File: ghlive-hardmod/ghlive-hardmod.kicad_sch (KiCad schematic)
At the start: 8 parts, among them IC1 LDL212D33R, J1 Conn_01x02, U2 ESP32-S3-WROOM-1

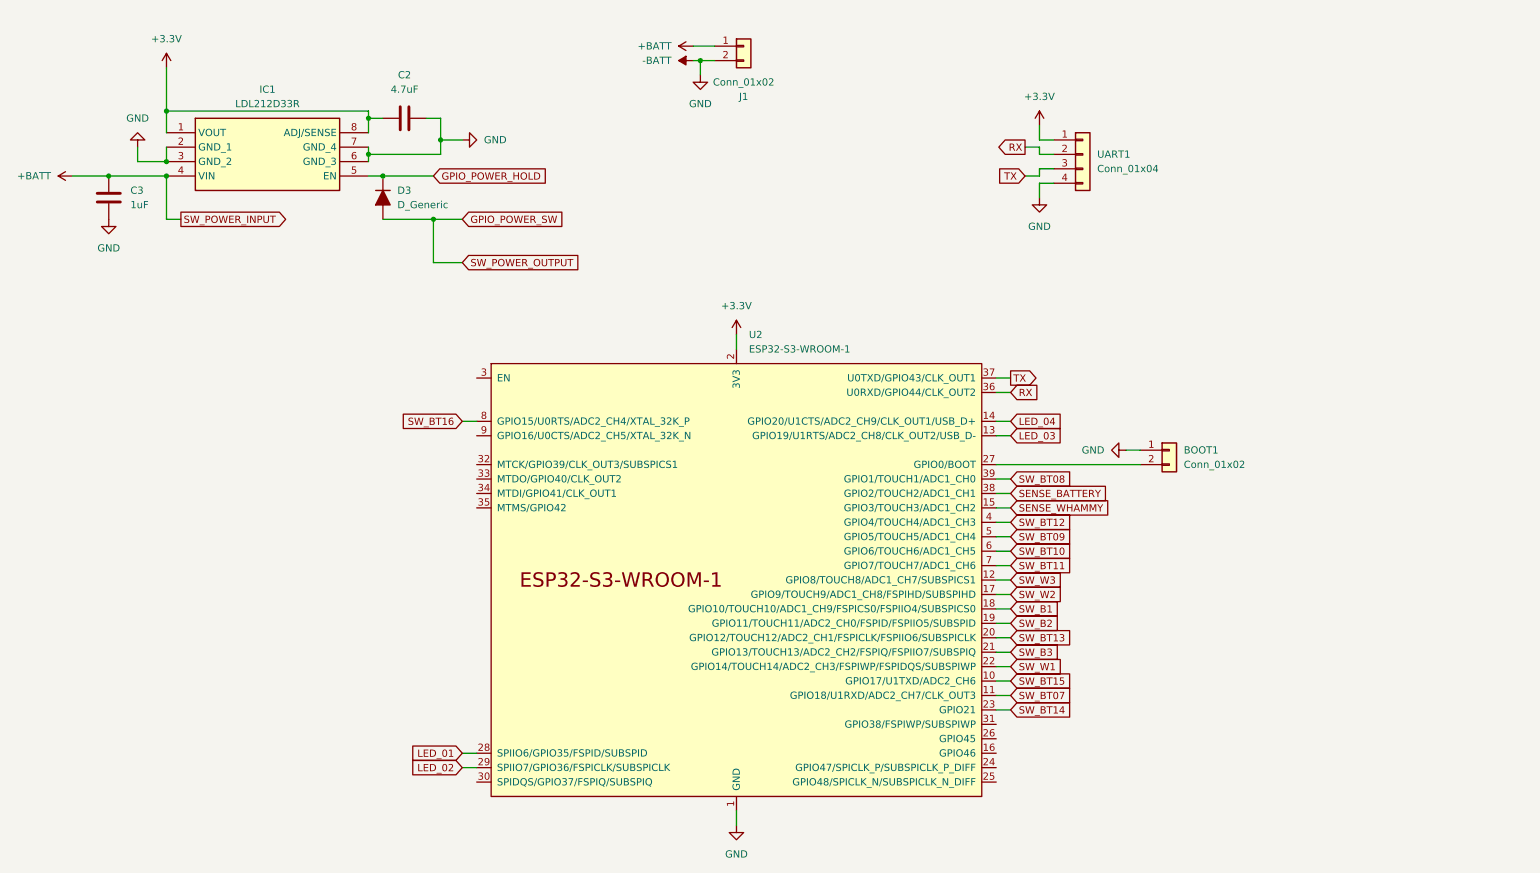
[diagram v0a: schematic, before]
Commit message: Wip schematic
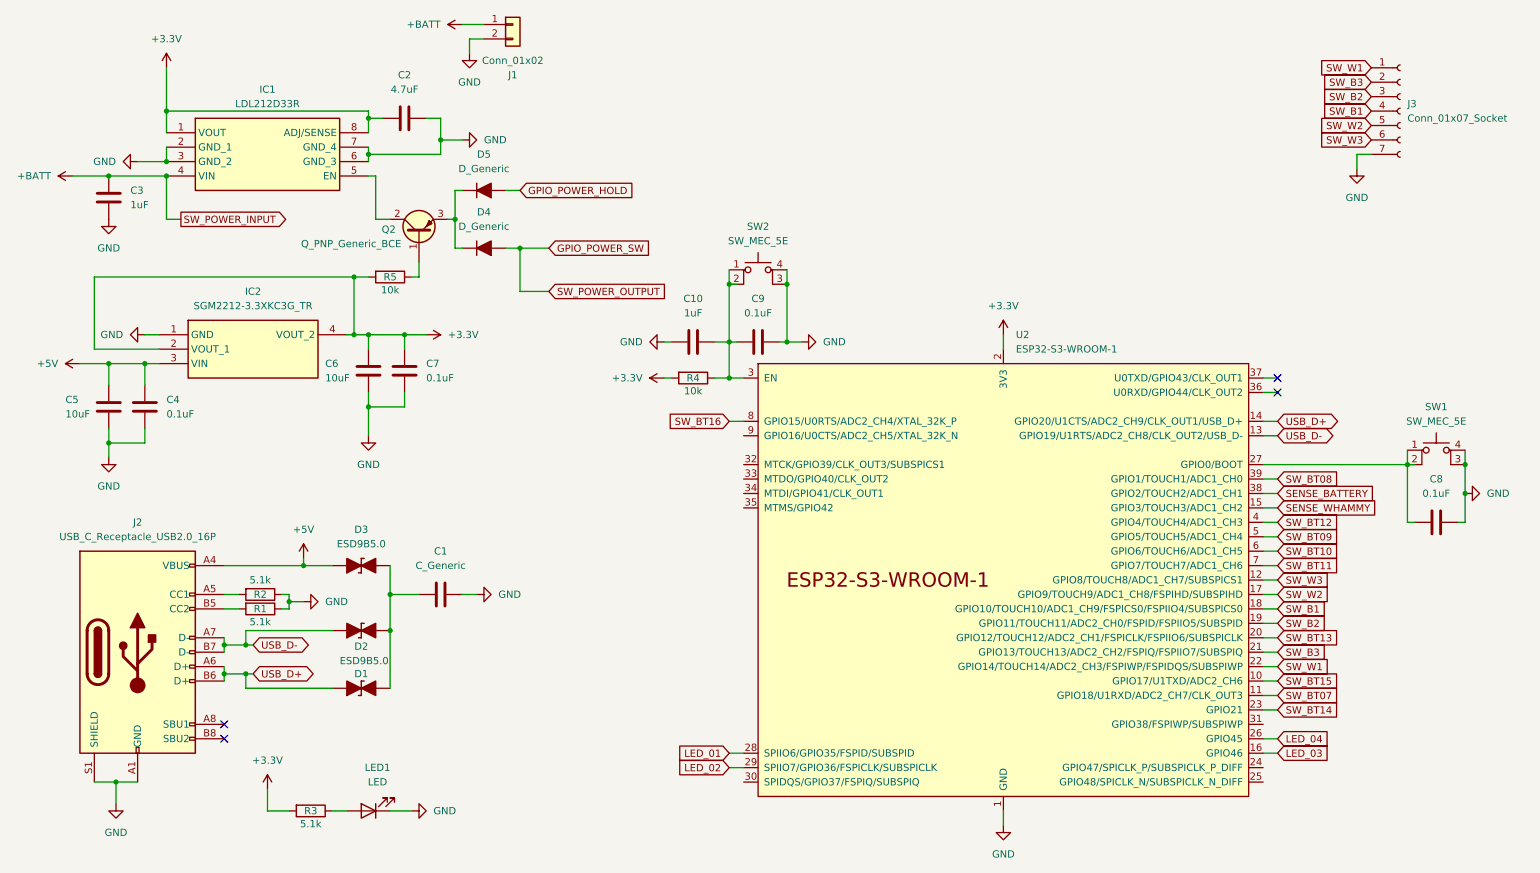
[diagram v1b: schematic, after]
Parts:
- removed BOOT1: Conn_01x02, symbol Connector_Generic:Conn_01x02
- removed UART1: Conn_01x04, symbol Connector_Generic:Conn_01x04
- added C1: C_Generic, symbol PCM_Capacitor_AKL:C_Generic
- added C10: 1uF, symbol PCM_Capacitor_AKL:C_Generic
- added C4, C7, C8, C9: 0.1uF, symbol PCM_Capacitor_AKL:C_Generic
- added C5, C6: 10uF, symbol PCM_Capacitor_AKL:C_Generic
- added D1, D2, D3: ESD9B5.0, symbol PCM_Diode_TVS_AKL:ESD9B5.0
- added D5: D_Generic, symbol PCM_Diode_AKL:D_Generic
- added IC2: SGM2212-3.3XKC3G_TR, symbol SGM2212-3_3XKC3G_TR:SGM2212-3.3XKC3G_TR
- added J2: USB_C_Receptacle_USB2.0_16P, symbol Connector:USB_C_Receptacle_USB2.0_16P
- added J3: Conn_01x07_Socket, symbol Connector:Conn_01x07_Socket
- added LED1: LED, symbol Device:LED
- added Q2: Q_PNP_Generic_BCE, symbol PCM_Transistor_BJT_AKL:Q_PNP_Generic_BCE
- added R1, R2, R3: 5.1k, symbol PCM_Resistor_AKL:R_Generic
- added R4, R5: 10k, symbol PCM_Resistor_AKL:R_Generic
- added SW1, SW2: SW_MEC_5E, symbol Switch:SW_MEC_5E
- IC1: footprint SOIC127P600X175-8N -> (none)
- U2: footprint PCM_Espressif:ESP32-S3-WROOM-1 -> (none)
- renumbered D3 to D4
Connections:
- net +3.3V: now also C6.2, C7.1, IC2.2 (VOUT_1), IC2.4 (VOUT_2), R3.2, R4.2, R5.2
- net GPIO_POWER_HOLD: now also D5.2 (A); no longer D4.1 (K), IC1.5 (EN)
- net LED_03: now also U2.16 (GPIO46); no longer U2.13 (GPIO19/U1RTS/ADC2_CH8/CLK_OUT2/USB_D-)
- net LED_04: now also U2.26 (GPIO45); no longer U2.14 (GPIO20/U1CTS/ADC2_CH9/CLK_OUT1/USB_D+)
- net SW_B1: now also J3.4 (Pin_4)
- net SW_B2: now also J3.3 (Pin_3)
- net SW_B3: now also J3.2 (Pin_2)
- net SW_W1: now also J3.1 (Pin_1)
- net SW_W2: now also J3.5 (Pin_5)
- net SW_W3: now also J3.6 (Pin_6)
- net at U2.27 (GPIO0/BOOT): now also C8.1, SW1.1, SW1.2
- net at U2.3 (EN): now also C10.1, C9.1, R4.1, SW2.1, SW2.2
- net -BATT renamed GND
- net GND: now also C1.2, C10.2, C4.2, C5.1, C6.1, C7.2, C8.2, C9.2, IC2.1 (GND), J2.A1 (GND), J2.A12 (GND), J2.B1 (GND), J2.B12 (GND), J2.S1 (SHIELD), J3.7 (Pin_7), LED1.1 (K), R1.1, R2.1, SW1.3 (K), SW1.4 (A), SW2.3 (K), SW2.4 (A)
- net RX: no longer names the net of U2.36 (U0RXD/GPIO44/CLK_OUT2)
- net TX: no longer names the net of U2.37 (U0TXD/GPIO43/CLK_OUT1)
- new net: IC1.5 (EN), Q2.2 (C)
- new net: C1.1, D1.1 (K), D2.1 (K), D3.1 (K)
- new net: D4.1 (K), D5.1 (K), Q2.3 (E)
- new net: J2.A5 (CC1), R2.2
- new net: Q2.1 (B), R5.1
- new net: J2.B5 (CC2), R1.2
- new net: LED1.2 (A), R3.1
- new net +5V: C4.1, C5.2, D3.2 (A), IC2.3 (VIN), J2.A4 (VBUS), J2.A9 (VBUS), J2.B4 (VBUS), J2.B9 (VBUS)
- new net USB_D+: D2.2 (A), J2.A6 (D+), J2.B6 (D+), U2.14 (GPIO20/U1CTS/ADC2_CH9/CLK_OUT1/USB_D+)
- new net USB_D-: D1.2 (A), J2.A7 (D-), J2.B7 (D-), U2.13 (GPIO19/U1RTS/ADC2_CH8/CLK_OUT2/USB_D-)
- no-connect marks 0 -> 4
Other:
- moved on the sheet: D4, J1, U2
